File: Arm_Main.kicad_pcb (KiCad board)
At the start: 2 copper layers, 100 x 110 mm, 33 parts, among them IC1 TLP559_F_, J1 Conn_01x03_Socket, J2 Conn_01x02_Pin, J4 Conn_01x03_Pin, J5 Conn_01x03_Pin, J6 Conn_01x03_Pin, SW2 SW_SPDT, U1 RASPBERRY_PI_ZERO_2_W, U2 TLP2531, U3 TLP2531

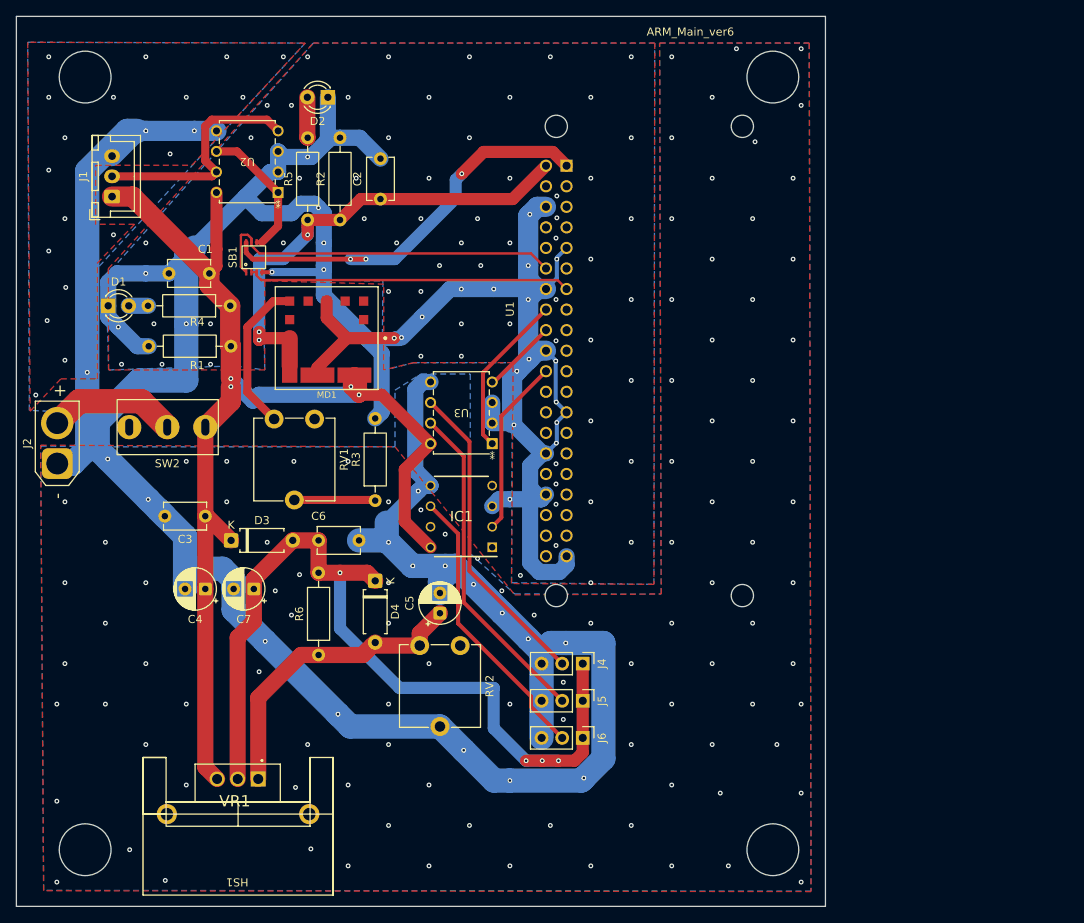
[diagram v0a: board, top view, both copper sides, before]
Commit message: Ver_7
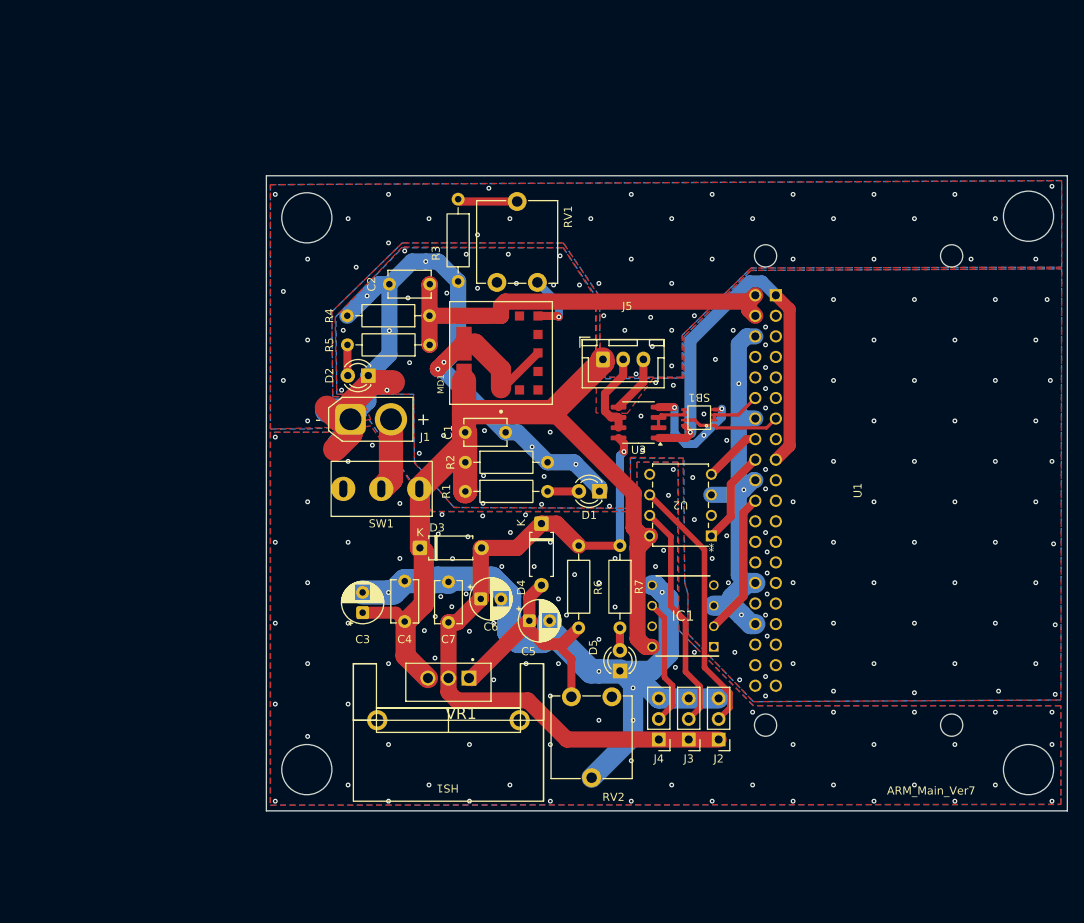
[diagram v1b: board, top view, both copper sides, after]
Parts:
- removed J6: Conn_01x03_Pin, Connector_PinHeader_2.54mm:PinHeader_1x03_P2.54mm_Vertical
- removed SW2: SW_SPDT, Togle_original:TogleSW3pin
- added D5: LED, LED_THT:LED_D3.0mm, F.Cu at (153.6, 120.9)
- added J3: Conn_01x03_Pin, Connector_PinHeader_2.54mm:PinHeader_1x03_P2.54mm_Vertical, F.Cu at (162.1, 129.4)
- added R7: 1k, Resistor_THT:R_Axial_DIN0207_L6.3mm_D2.5mm_P10.16mm_Horizontal, F.Cu at (153.6, 105.4)
- added SW1: SW_SPDT, Togle_original:TogleSW3pin, F.Cu at (124.1, 98.4)
- C3: value 0.1u -> 100u; footprint Capacitor_THT:C_Disc_D5.1mm_W3.2mm_P5.00mm -> Capacitor_THT:CP_Radial_D5.0mm_P2.50mm
- C4: value 100u -> 0.1u; footprint Capacitor_THT:CP_Radial_D5.0mm_P2.50mm -> Capacitor_THT:C_Disc_D5.1mm_W3.2mm_P5.00mm
- C6: value 0.1u -> 47u; footprint Capacitor_THT:C_Disc_D5.1mm_W3.2mm_P5.00mm -> Capacitor_THT:CP_Radial_D5.0mm_P2.50mm
- C7: value 47u -> 0.1u; footprint Capacitor_THT:CP_Radial_D5.0mm_P2.50mm -> Capacitor_THT:C_Disc_D5.1mm_W3.2mm_P5.00mm
- J1: value Conn_01x03_Socket -> Conn_01x02_Pin; footprint Connector_JST:JST_XH_B3B-XH-A_1x03_P2.50mm_Vertical -> Connector_AMASS:AMASS_XT30U-F_1x02_P5.0mm_Vertical
- J2: value Conn_01x02_Pin -> Conn_01x03_Pin; footprint Connector_AMASS:AMASS_XT30U-F_1x02_P5.0mm_Vertical -> Connector_PinHeader_2.54mm:PinHeader_1x03_P2.54mm_Vertical
- J5: value Conn_01x03_Pin -> Conn_01x03_Socket; footprint Connector_PinHeader_2.54mm:PinHeader_1x03_P2.54mm_Vertical -> Connector_JST:JST_XH_B3B-XH-A_1x03_P2.50mm_Vertical
- R1: value 20k -> 2k
- R2: value 1.2k -> 20k
- R4: value 2k -> 1.2k
- RV1, RV2: value R_Potentiometer_Trim -> R_Trim
- U3: value TLP2531 -> ADuM121N; footprint ul_TLP2531:U_DIP8_11-10C4S_TOS -> Package_SO:SOIC-8_3.9x4.9mm_P1.27mm
- VR1: footprint NJM317:TO254P1054X470X1955-3 -> Njm317_original:TO254P1054X470X1955-3
- moved J2 88.6 mm to (165.8, 129.4), turned to 180 degrees
- moved U2 68.3 mm to (164.9, 104.2)
- moved D1 64.9 mm to (151.1, 98.7), turned to 180 degrees
- moved SB1 58.5 mm to (163.4, 89.6), turned to 180 degrees
- moved J5 42.3 mm to (151.5, 82.4), turned to 0 degrees
- moved J1 40.3 mm to (120.3, 89.8), turned to 0 degrees
- moved R3 38.6 mm to (133.6, 62.6), turned to -90 degrees
- moved C1 37.2 mm to (134.5, 91.4), turned to 0 degrees
- moved RV1 36.7 mm to (143.4, 72.9), turned to 90 degrees
- moved D2 34.8 mm to (122.5, 84.4)
- moved R1 34.1 mm to (134.5, 98.7), turned to 0 degrees
- moved R2 33.7 mm to (134.5, 95.1), turned to 0 degrees
- moved R6 32.3 mm to (148.5, 115.6)
- moved U1 30.4 mm to (183.1, 98.6)
- moved IC1 30.0 mm to (161.4, 114.1)
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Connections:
- C1 pad 1: Net-(D3-K) -> Batte
- C2 pad 1: Net-(MD1-SENSE) -> +5V_Digital
- C3 pad 1: Net-(D3-K) -> Batte
- C4 pad 1: Net-(D3-K) -> Batte
- C6 pad 1: Net-(D3-A) -> +5V_Analog
- C7 pad 1: Net-(D3-A) -> +5V_Analog
- D3 pad 1: Net-(D3-K) -> Batte
- D3 pad 2: Net-(D3-A) -> +5V_Analog
- D4 pad 1: Net-(D3-A) -> +5V_Analog
- IC1 pad 8: Net-(D3-K) -> Batte
- J1 pad 1: Net-(D3-K) -> GNDA
- J2 pad 1: GNDA -> +5V_Analog
- J2 pad 2: +BATT -> Net-(J2-Pin_2)
- J4 pad 1: Net-(D3-A) -> +5V_Analog
- J4 pad 2: Net-(J4-Pin_2) -> Net-(IC1-COLLECTER)
- J5 pad 1: Net-(D3-A) -> Batte
- MD1 pad 2: Net-(D3-K) -> Batte
- MD1 pad 4: Net-(MD1-SENSE) -> +5V_Digital
- MD1 pad 5: Net-(MD1-SENSE) -> +5V_Digital
- R1 pad 1: Net-(D3-K) -> Batte
- R1 pad 2: GNDA -> Net-(D1-A)
- R2 pad 1: Net-(MD1-SENSE) -> Batte
- R4 pad 1: Net-(D3-K) -> +5V_Digital
- R4 pad 2: Net-(D1-A) -> GNDA
- R5 pad 1: Net-(MD1-SENSE) -> +5V_Digital
- R6 pad 2: Net-(D3-A) -> +5V_Analog
- U1 pad 12: Net-(SB1-G') -> Net-(SB1-A1)
- U1 pad 13: Net-(SB1-A1) -> Net-(SB1-G')
- U1 pad 17: unconnected-(U1-3V3_17-Pad17) -> Net-(SB1-Vcc)
- U1 pad 2: Net-(MD1-SENSE) -> +5V_Digital
- U1 pad 4: unconnected-(U1-5V_4-Pad4) -> +5V_Digital
- U2 pad 1: Net-(SB1-A2) -> Net-(U1-GPIO24/GPIO_GEN5)
- U2 pad 4: Net-(J1-Pin_2) -> Net-(U1-GPIO23/GPIO_GEN4)
- U2 pad 6: Net-(SB1-A2) -> Net-(J2-Pin_2)
- U2 pad 7: Net-(J1-Pin_2) -> Net-(J3-Pin_2)
- U2 pad 8: Net-(D3-K) -> Batte
- U3 pad 1: Net-(U1-GPIO23/GPIO_GEN4) -> Net-(SB1-Vcc)
- U3 pad 2: GNDA -> Net-(SB1-A2)
- U3 pad 3: GNDA -> Net-(SB1-A2)
- U3 pad 4: Net-(U1-GPIO24/GPIO_GEN5) -> GNDA
- U3 pad 6: Net-(J4-Pin_2) -> Net-(J5-Pin_2)
- U3 pad 8: Net-(D3-K) -> +5V_Analog
- VR1 pad 2: Net-(D3-A) -> +5V_Analog
- VR1 pad 3: Net-(D3-K) -> Batte
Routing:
- net GNDA: track 525.8 -> 280.8 mm, vias 222 -> 239
- net Net-(D3-K): track 147.4 -> 0.00 mm, vias 4 -> 0
- net Batte: track 0.00 -> 113.7 mm
- net Net-(D3-A): track 108.9 -> 0.00 mm, vias 4 -> 0
- net +5V_Analog: track 0.00 -> 89.3 mm, vias 0 -> 1
- net Net-(MD1-SENSE): track 60.5 -> 0.00 mm, vias 3 -> 0
- net +5V_Digital: track 0.00 -> 57.1 mm
- net Net-(J4-Pin_2): track 39.0 -> 0.00 mm
- net Net-(SB1-A1): track 40.0 -> 6.59 mm
- net Net-(SB1-G'): track 44.8 -> 12.2 mm
- net Net-(J2-Pin_2): track 0.00 -> 32.4 mm
- net Net-(J5-Pin_2): track 41.1 -> 10.6 mm
- net Net-(J3-Pin_2): track 0.00 -> 28.3 mm
- net Net-(J1-Pin_2): track 29.3 -> 9.10 mm
- net Net-(IC1-COLLECTER): track 35.4 -> 15.7 mm
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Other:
- board size 100 x 110 mm -> 99 x 78.5 mm
- board text added: "ARM_Main_Ver7"
- board text removed: "ARM_Main_ver6"
